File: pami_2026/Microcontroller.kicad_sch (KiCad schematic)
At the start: 11 parts, among them U1 ESP32-WROOM-E

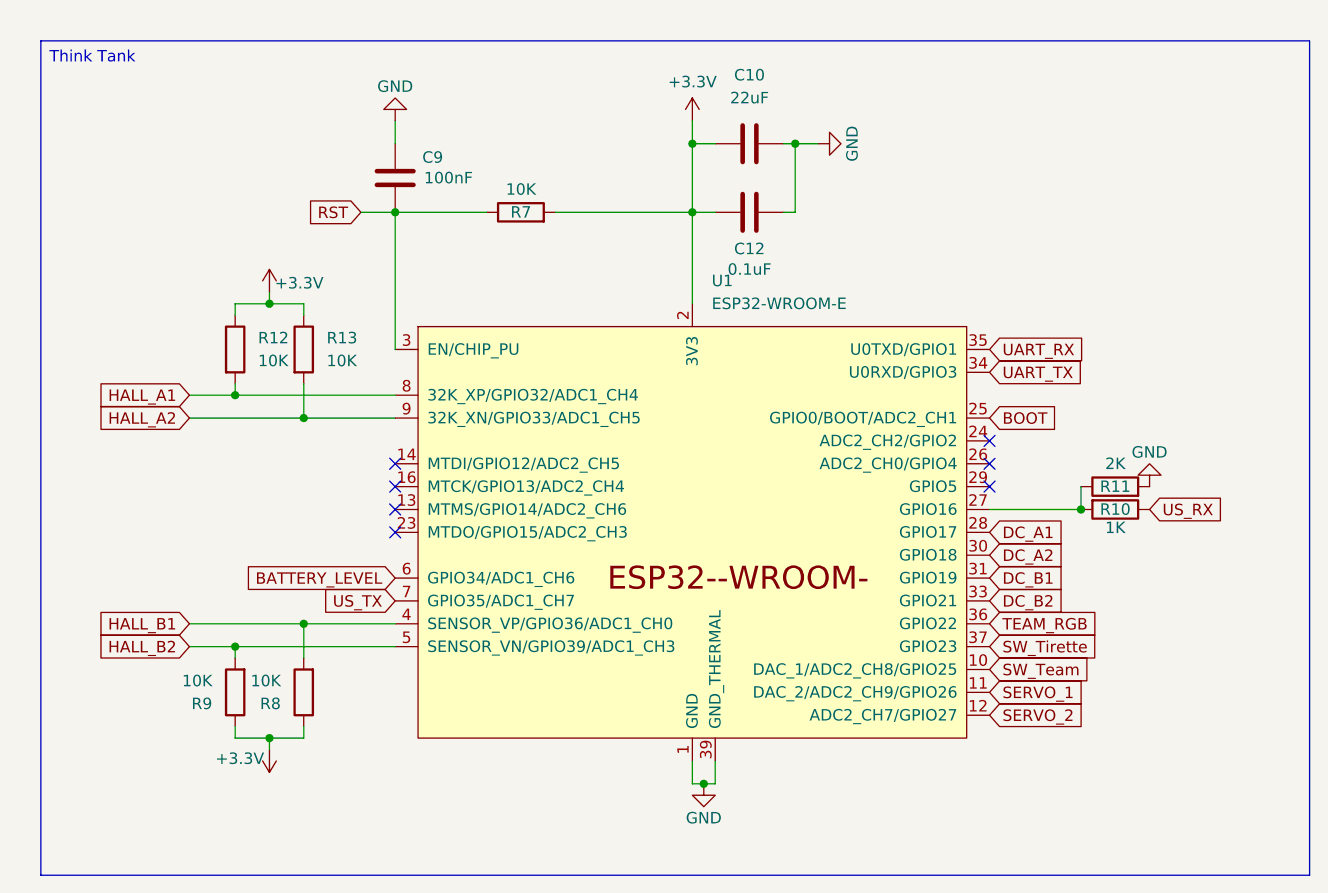
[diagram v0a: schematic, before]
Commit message: FEAT : Routing
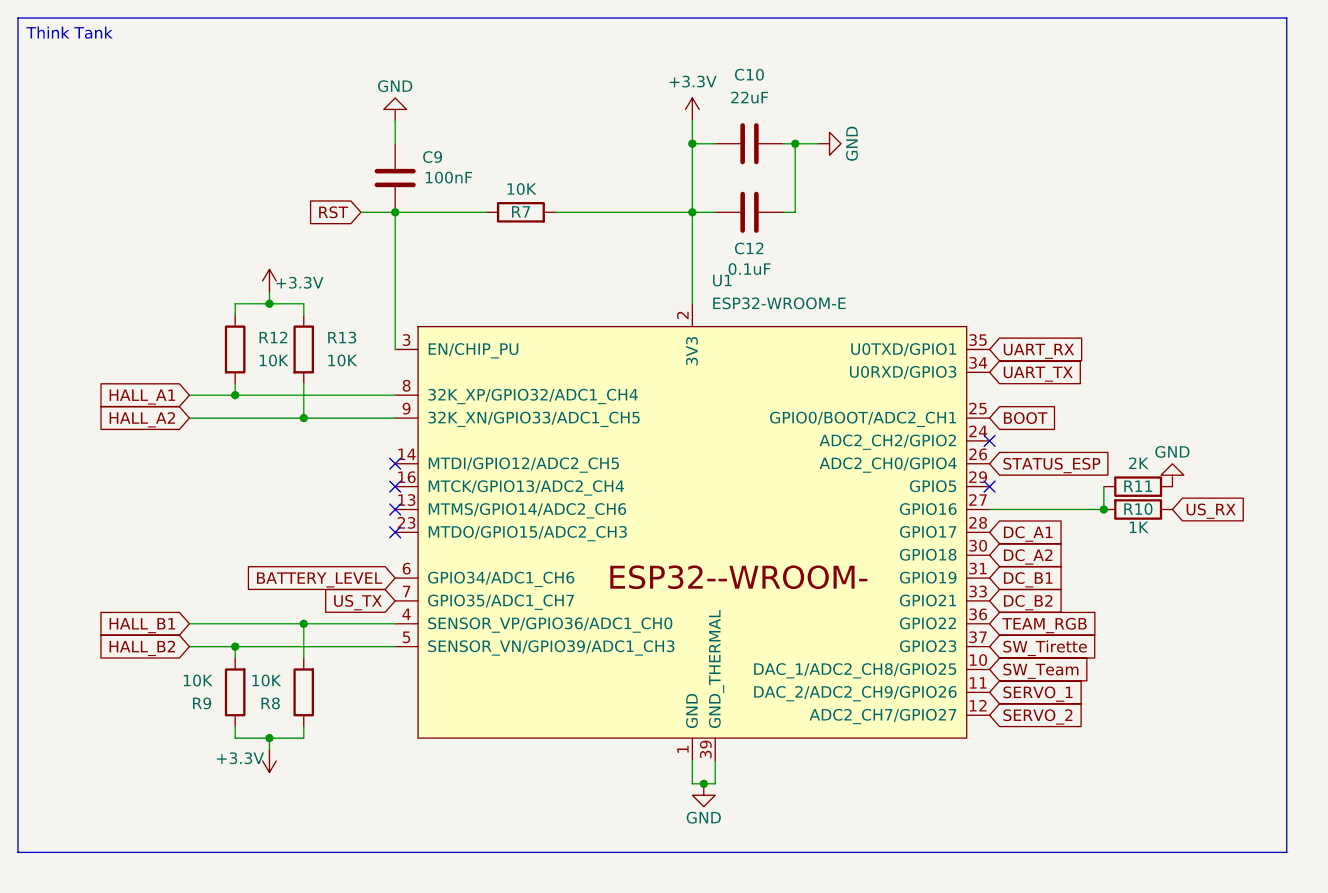
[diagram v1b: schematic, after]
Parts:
- U1: footprint PCM_Espressif:ESP32-WROOM-32E -> lib:ESP32-WROOM-32E
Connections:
- net STATUS_ESP: now reaches U1.26 (ADC2_CH0/GPIO4)
- no-connect marks 7 -> 6
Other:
- moved on the sheet: R10, R11
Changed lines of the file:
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@@
 	(text_box "Think Tank"
 		(exclude_from_sim no)
-		(at 76.2 52.07 0)
+		(at 73.66 49.53 0)
 		(size 140.97 92.71)
 		(margins 0.9525 0.9525 0.9525 0.9525)
@@
 	)
 	(junction
-		(at 191.77 104.14)
+		(at 194.31 104.14)
 		(diameter 0)
 		(color 0 0 0 0)
@@
 	)
 	(no_connect
-		(at 181.61 99.06)
-	)
-	(no_connect
 		(at 115.57 99.06)
 	)
@@
 	(wire
 		(pts
-			(xy 191.77 104.14) (xy 191.77 101.6)
+			(xy 194.31 104.14) (xy 194.31 101.6)
+		)
+		(stroke
+			(width 0)
+			(type default)
+		)
+	)
+	(wire
+		(pts
+			(xy 181.61 104.14) (xy 194.31 104.14)
 		)
 		(stroke
@@
 		(pts
 			(xy 101.6 80.01) (xy 101.6 81.28)
-		)
-		(stroke
-			(width 0)
-			(type default)
-		)
-	)
-	(wire
-		(pts
-			(xy 181.61 104.14) (xy 191.77 104.14)
 		)
 		(stroke
@@
 		)
 	)
+	(global_label "STATUS_ESP"
+		(shape input)
+		(at 181.61 99.06 0)
+		(fields_autoplaced yes)
+		(effects
+			(font
+				(size 1.27 1.27)
+			)
+			(justify left)
+		)
+		(property "Intersheetrefs" "${INTERSHEET_REFS}"
+			(at 195.9646 99.06 0)
+			(effects
+				(font
+					(size 1.27 1.27)
+				)
+				(justify left)
+				(hide yes)
+			)
+		)
+	)
 	(global_label "SW_Team"
 		(shape input)
@@
 	(global_label "US_RX"
 		(shape input)
-		(at 199.39 104.14 0)
+		(at 201.93 104.14 0)
 		(fields_autoplaced yes)
 		(effects
@@
 		)
 		(property "Intersheetrefs" "${INTERSHEET_REFS}"
-			(at 208.3623 104.14 0)
+			(at 210.9023 104.14 0)
 			(effects
 				(font
@@
 	(symbol
 		(lib_id "Device:R")
-		(at 195.58 104.14 270)
+		(at 198.12 104.14 270)
 		(unit 1)
 		(exclude_from_sim no)
@@
 		(dnp no)
 		(property "Reference" "R10"
-			(at 195.58 104.14 90)
+			(at 198.12 104.14 90)
 			(effects
 				(font
@@
 		)
 		(property "Value" "1K"
-			(at 195.58 106.172 90)
+			(at 198.12 106.172 90)
 			(effects
 				(font
@@
 		)
 		(property "Footprint" "Resistor_SMD:R_0603_1608Metric"
-			(at 195.58 102.362 90)
+			(at 198.12 102.362 90)
 			(effects
 				(font
@@
 		)
 		(property "Datasheet" "~"
-			(at 195.58 104.14 0)
+			(at 198.12 104.14 0)
 			(effects
 				(font
@@
 		)
 		(property "Description" "Resistor"
-			(at 195.58 104.14 0)
+			(at 198.12 104.14 0)
 			(effects
 				(font
@@
 	(symbol
 		(lib_id "PCM_SparkFun-PowerSymbol:GND")
-		(at 199.39 101.6 180)
+		(at 201.93 101.6 180)
 		(unit 1)
 		(exclude_from_sim no)
@@
 		(fields_autoplaced yes)
 		(property "Reference" "#PWR050"
-			(at 199.39 95.25 0)
+			(at 201.93 95.25 0)
 			(effects
 				(font
@@
 		)
 		(property "Value" "GND"
-			(at 199.39 97.79 0)
+			(at 201.93 97.79 0)
 			(do_not_autoplace yes)
 			(effects
@@
 		)
 		(property "Footprint" ""
-			(at 199.39 101.6 0)
+			(at 201.93 101.6 0)
 			(effects
 				(font
@@
 		)
 		(property "Datasheet" ""
-			(at 199.39 101.6 0)
+			(at 201.93 101.6 0)
 			(effects
 				(font
@@
 		)
 		(property "Description" "Power symbol creates a global label with name \"GND\" , ground"
-			(at 199.39 92.71 0)
+			(at 201.93 92.71 0)
 			(effects
 				(font
@@
 	(symbol
 		(lib_id "Device:R")
-		(at 195.58 101.6 90)
+		(at 198.12 101.6 90)
 		(unit 1)
 		(exclude_from_sim no)
@@
 		(dnp no)
 		(property "Reference" "R11"
-			(at 195.58 101.6 90)
+			(at 198.12 101.6 90)
 			(effects
 				(font
@@
 		)
 		(property "Value" "2K"
-			(at 195.58 99.06 90)
+			(at 198.12 99.06 90)
 			(effects
 				(font
@@
 		)
 		(property "Footprint" "Resistor_SMD:R_0603_1608Metric"
-			(at 195.58 103.378 90)
+			(at 198.12 103.378 90)
 			(effects
 				(font
@@
 		)
 		(property "Datasheet" "~"
-			(at 195.58 101.6 0)
+			(at 198.12 101.6 0)
 			(effects
 				(font
@@
 		)
 		(property "Description" "Resistor"
-			(at 195.58 101.6 0)
+			(at 198.12 101.6 0)
 			(effects
 				(font
@@
 			)
 		)
-		(property "Footprint" "PCM_Espressif:ESP32-WROOM-32E"
+		(property "Footprint" "lib:ESP32-WROOM-32E"
 			(at 148.59 142.24 0)
 			(effects
